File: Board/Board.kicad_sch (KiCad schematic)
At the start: 4 parts, among them J2 Conn_02x25_Odd_Even

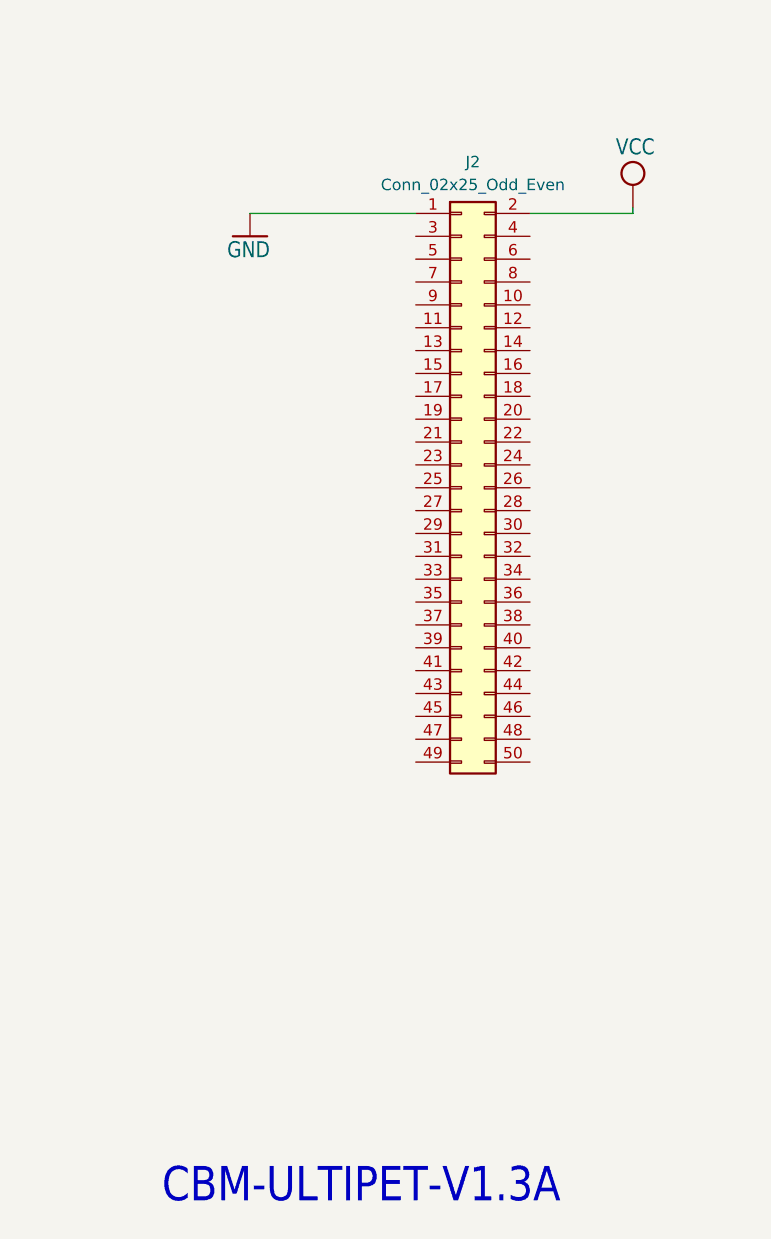
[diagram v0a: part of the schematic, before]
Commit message: more work on the frontpanel
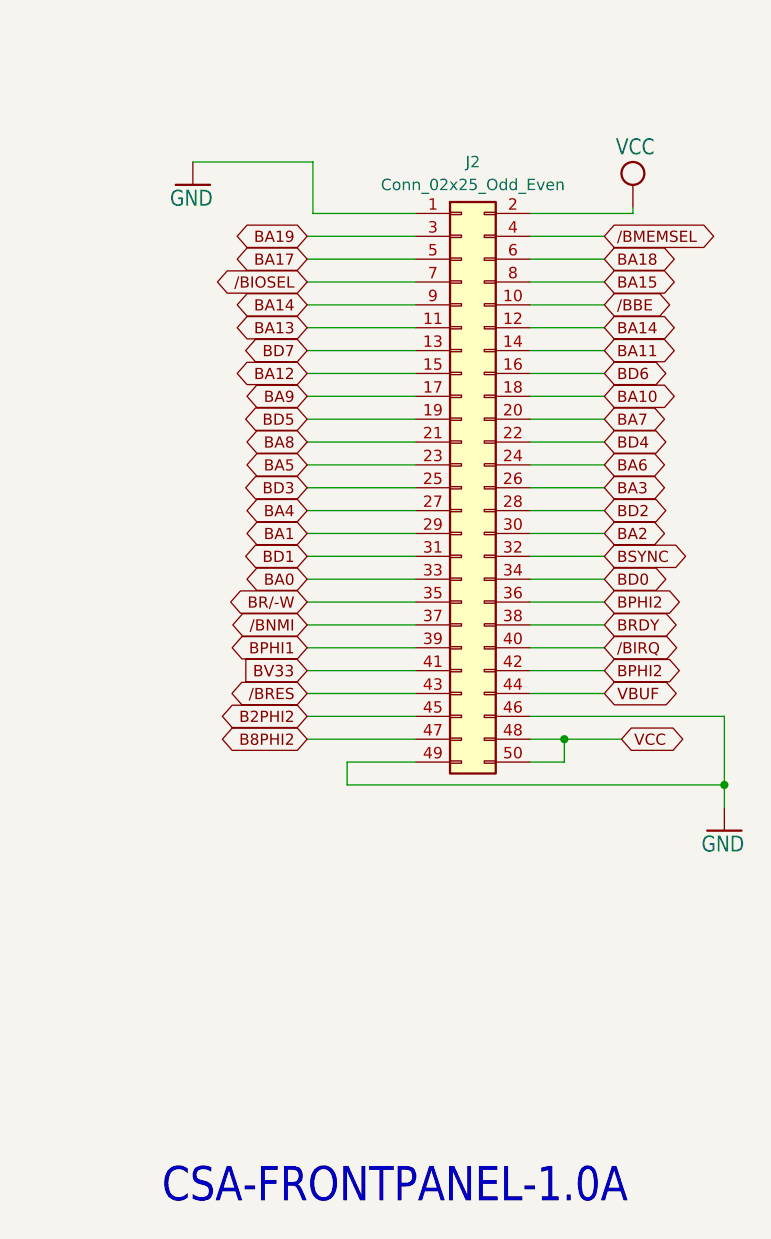
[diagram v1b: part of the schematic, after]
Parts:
- C1, C2: LCSC (none) -> C96123
- J2: LCSC (none) -> C30006
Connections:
- net /BBE: now also J2.10 (Pin_10)
- net /BIOSEL: now also J2.7 (Pin_7)
- net /BIRQ: now also J2.40 (Pin_40)
- net /BMEMSEL: now also J2.4 (Pin_4)
- net /BNMI: now also J2.37 (Pin_37)
- net /BRES: now also J2.43 (Pin_43)
- net B2PHI2: now also J2.45 (Pin_45)
- net B8PHI2: now also J2.47 (Pin_47)
- net BA0: now also J2.33 (Pin_33)
- net BA1: now also J2.29 (Pin_29)
- net BA10: now also J2.18 (Pin_18)
- net BA11: now also J2.14 (Pin_14)
- net BA12: now also J2.15 (Pin_15)
- net BA13: now also J2.11 (Pin_11)
- net BA14: now also J2.12 (Pin_12), J2.9 (Pin_9)
- net BA15: now also J2.8 (Pin_8)
- net BA17: now also J2.5 (Pin_5)
- net BA18: now also J2.6 (Pin_6)
- net BA19: now also J2.3 (Pin_3)
- net BA2: now also J2.30 (Pin_30)
- net BA3: now also J2.26 (Pin_26)
- net BA4: now also J2.27 (Pin_27)
- net BA5: now also J2.23 (Pin_23)
- net BA6: now also J2.24 (Pin_24)
- net BA7: now also J2.20 (Pin_20)
- net BA8: now also J2.21 (Pin_21)
- net BA9: now also J2.17 (Pin_17)
- net BD0: now also J2.34 (Pin_34)
- net BD1: now also J2.31 (Pin_31)
- net BD2: now also J2.28 (Pin_28)
- net BD3: now also J2.25 (Pin_25)
- net BD4: now also J2.22 (Pin_22)
- net BD5: now also J2.19 (Pin_19)
- net BD6: now also J2.16 (Pin_16)
- net BD7: now also J2.13 (Pin_13)
- net BPHI1: now also J2.39 (Pin_39)
- net BPHI2: now also J2.36 (Pin_36), J2.42 (Pin_42)
- net BR/-W: now also J2.35 (Pin_35)
- net BRDY: now also J2.38 (Pin_38)
- net BSYNC: now also J2.32 (Pin_32)
- net BV33: now also J2.41 (Pin_41)
- net GND: now also J2.46 (Pin_46), J2.49 (Pin_49)
- net VBUF: now also J2.44 (Pin_44)
- net VCC: now also J2.48 (Pin_48), J2.50 (Pin_50)
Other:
- note added: "CSA-FRONTPANEL-1.0A"
- note removed: "CBM-ULTIPET-V1.3A"
